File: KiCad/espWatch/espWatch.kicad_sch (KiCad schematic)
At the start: 8 parts, among them U2 NodeMCU_1.0_(ESP-12E), U3 1.8" TFT ST7735, U4 RTC DS3231, U5 KY-040_Rotary_Encoder

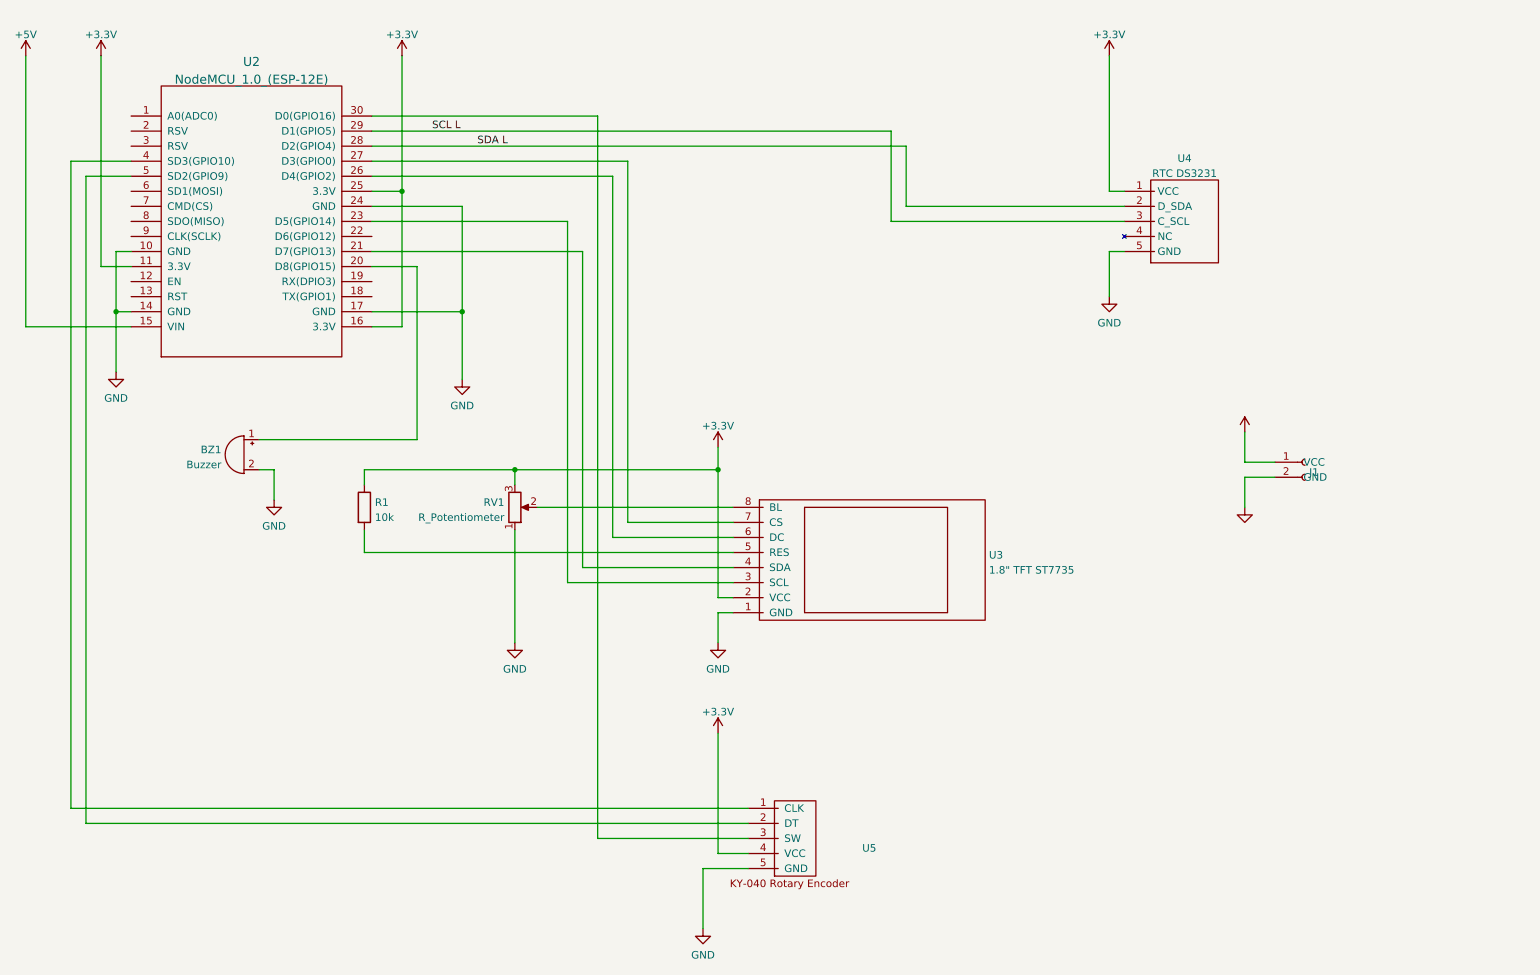
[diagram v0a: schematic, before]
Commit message: new schematics for esp
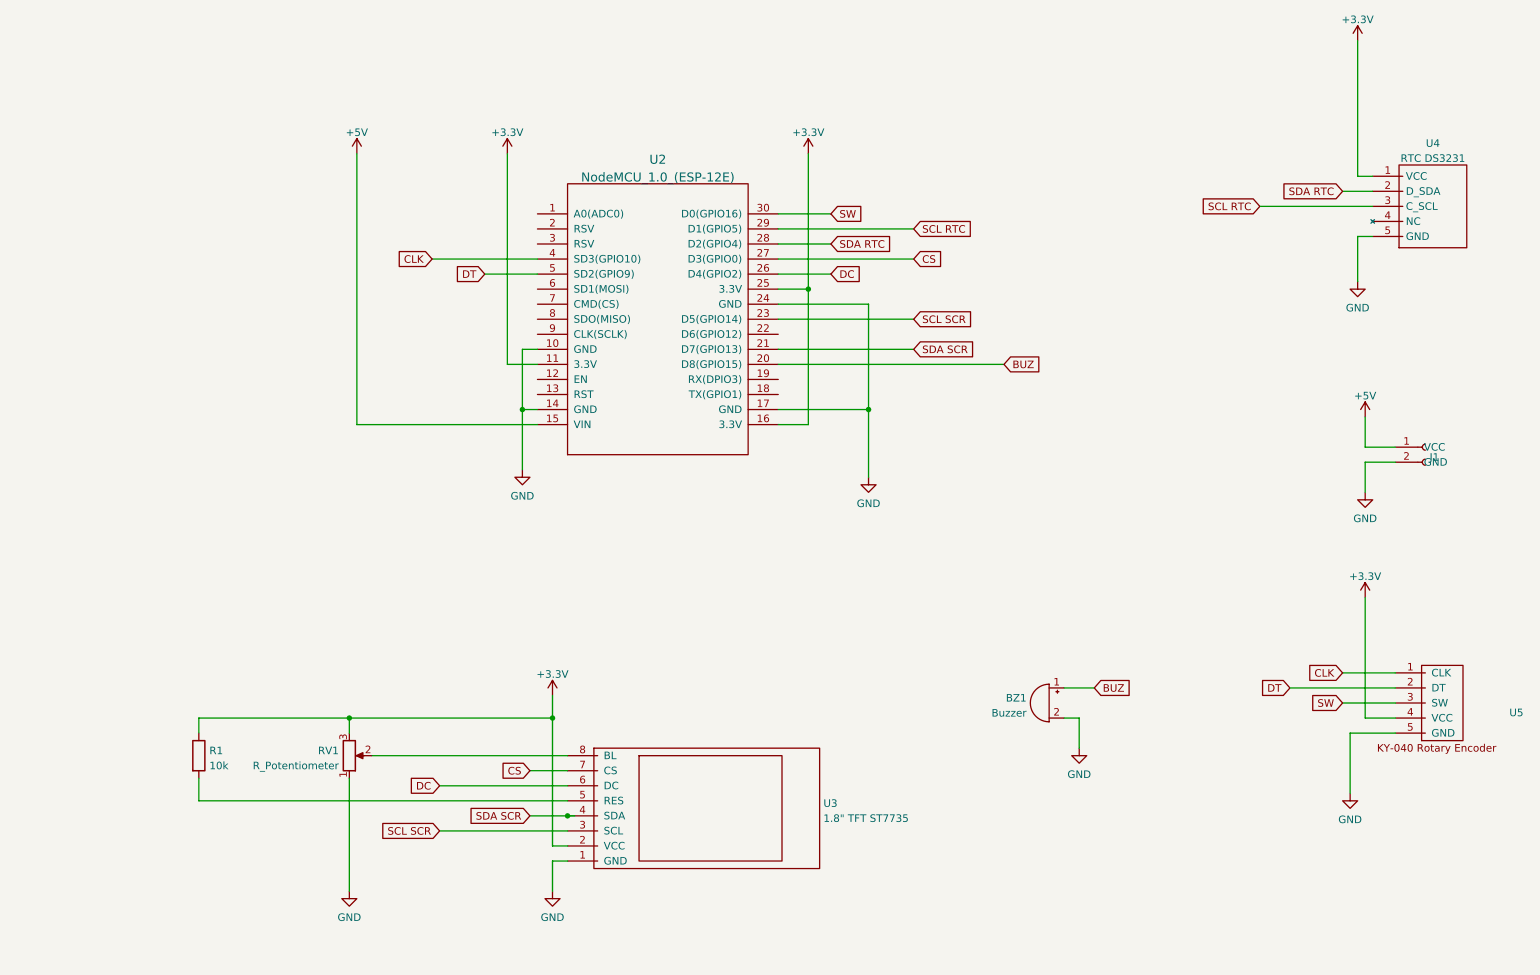
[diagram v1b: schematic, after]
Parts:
- J1: value (none) -> 2-pin_power_input_header; footprint (none) -> My_Headers:2-pin_power_input_header_larger_pads
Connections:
- net BUZ: now reaches BZ1.1 (-), U2.20 (D8(GPIO15))
- net SDA SCR: now reaches U2.21 (D7(GPIO13)), U3.4 (SDA)
- net SCL SCR: now reaches U2.23 (D5(GPIO14)), U3.3 (SCL)
- net DC: now reaches U2.26 (D4(GPIO2)), U3.6 (DC)
- net CS: now reaches U2.27 (D3(GPIO0)), U3.7 (CS)
- net SW: now reaches U2.30 (D0(GPIO16)), U5.3 (SW)
- net CLK: now reaches U2.4 (SD3(GPIO10)), U5.1 (CLK)
- net DT: now reaches U2.5 (SD2(GPIO9)), U5.2 (DT)
- net SCL L renamed SCL RTC
- net SDA L renamed SDA RTC
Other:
- moved on the sheet: BZ1, J1, R1, RV1, U2, U3, U4, U5
